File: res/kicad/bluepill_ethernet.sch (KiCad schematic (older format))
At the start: 12 parts, among them J2 Conn_01x03, U1 BluePill_STM32F103C, U2 93C46, U3 WIZ850io

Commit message: Add button to kicad circuit for 'factory reset' the configuration (delete eeprom)
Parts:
- added SW?: SW_Push, symbol switches:SW_Push
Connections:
- wire segments 100 -> 104
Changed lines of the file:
@@
 	5600 1200 5600 1500
+Wire Wire Line
+	3050 900  2450 900
 Wire Wire Line
 	3050 900  3750 900
@@
 Wire Wire Line
 	4300 2350 4300 2550
-Wire Wire Line
-	2150 900  3050 900
+$Comp
+L switches:SW_Push SW?
+U 1 1 5ADFA2DD
+P 2450 2500
+F 0 "SW?" V 2404 2648 50  0000 L CNN
+F 1 "SW_Push" V 2495 2648 50  0000 L CNN
+F 2 "" H 2450 2700 50  0001 C CNN
+F 3 "" H 2450 2700 50  0001 C CNN
+	1    2450 2500
+	0    1    1    0
+$EndComp
+Wire Wire Line
+	2550 2950 2450 2950
+Wire Wire Line
+	2450 2950 2450 2700
+Wire Wire Line
+	2450 2300 2450 900
+Connection ~ 2450 900
+Wire Wire Line
+	2450 900  2150 900
 $EndSCHEMATC

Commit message: Revision 2.0
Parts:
- added D1, D2, D3: LED, LEDs:LED_D3.0mm, symbol device:LED
- added J1: HEADER-1x20, Pin_Headers:Pin_Header_Straight_1x20_Pitch2.54mm, symbol connectors:HEADER-1x20
- added R2, R3, R4, R5, R6: R, Resistors_THT:R_Axial_DIN0204_L3.6mm_D1.6mm_P5.08mm_Horizontal, symbol device:R
- SW1: renamed from SW?; footprint (none) -> Buttons_Switches_THT:SW_PUSH_6mm
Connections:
- wire segments 104 -> 125
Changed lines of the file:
@@
 	4300 2350 4300 2550
 $Comp
-L switches:SW_Push SW?
+L switches:SW_Push SW1
 U 1 1 5ADFA2DD
 P 2450 2500
-F 0 "SW?" V 2404 2648 50  0000 L CNN
+F 0 "SW1" V 2404 2648 50  0000 L CNN
 F 1 "SW_Push" V 2495 2648 50  0000 L CNN
-F 2 "" H 2450 2700 50  0001 C CNN
+F 2 "Buttons_Switches_THT:SW_PUSH_6mm" H 2450 2700 50  0001 C CNN
 F 3 "" H 2450 2700 50  0001 C CNN
 	1    2450 2500
@@
 Wire Wire Line
 	2450 900  2150 900
+$Comp
+L connectors:HEADER-1x20 J1
+U 1 1 5B103221
+P 4450 3500
+F 0 "J1" H 4578 3536 60  0000 L CNB
+F 1 "HEADER-1x20" H 4578 3445 40  0000 L CNN
+F 2 "Pin_Headers:Pin_Header_Straight_1x20_Pitch2.54mm" H 4450 3500 60  0001 C CNN
+F 3 "" H 4450 3500 60  0001 C CNN
+F 4 "-" H 4400 4650 40  0001 L BNN "Part"
+F 5 "Connector" H 4400 4750 40  0001 L BNN "Family"
+	1    4450 3500
+	1    0    0    -1
+$EndComp
+Connection ~ 4300 2550
+Connection ~ 4300 2650
+Connection ~ 4300 2750
+$Comp
+L device:R R3
+U 1 1 5B105160
+P 3600 2850
+F 0 "R3" V 3680 2850 50  0000 C CNN
+F 1 "R" V 3600 2850 50  0000 C CNN
+F 2 "Resistors_THT:R_Axial_DIN0204_L3.6mm_D1.6mm_P5.08mm_Horizontal" V 3530 2850 50  0001 C CNN
+F 3 "" H 3600 2850 50  0001 C CNN
+	1    3600 2850
+	1    0    0    -1
+$EndComp
+$Comp
+L device:R R2
+U 1 1 5B105A17
+P 3500 2850
+F 0 "R2" V 3580 2850 50  0000 C CNN
+F 1 "R" V 3500 2850 50  0000 C CNN
+F 2 "Resistors_THT:R_Axial_DIN0204_L3.6mm_D1.6mm_P5.08mm_Horizontal" V 3430 2850 50  0001 C CNN
+F 3 "" H 3500 2850 50  0001 C CNN
+	1    3500 2850
+	1    0    0    -1
+$EndComp
+Wire Wire Line
+	3600 3050 3600 3000
+Wire Wire Line
+	3500 3150 3500 3000
+Wire Wire Line
+	4300 2550 3600 2550
+Wire Wire Line
+	3600 2550 3600 2700
+Wire Wire Line
+	3500 2700 3500 2550
+Wire Wire Line
+	3500 2550 3600 2550
+Connection ~ 3600 2550
+Wire Wire Line
+	3600 3050 4300 3050
+Connection ~ 4300 3050
+Wire Wire Line
+	3500 3150 4300 3150
+Connection ~ 4300 3150
+$Comp
+L device:LED D1
+U 1 1 5B11D9D9
+P 1100 4350
+F 0 "D1" V 1138 4233 50  0000 R CNN
+F 1 "LED" V 1047 4233 50  0000 R CNN
+F 2 "LEDs:LED_D3.0mm" H 1100 4350 50  0001 C CNN
+F 3 "" H 1100 4350 50  0001 C CNN
+	1    1100 4350
+	0    -1   -1   0
+$EndComp
+$Comp
+L device:LED D2
+U 1 1 5B11DDF6
+P 1350 4350
+F 0 "D2" V 1388 4233 50  0000 R CNN
+F 1 "LED" V 1297 4233 50  0000 R CNN
+F 2 "LEDs:LED_D3.0mm" H 1350 4350 50  0001 C CNN
+F 3 "" H 1350 4350 50  0001 C CNN
+	1    1350 4350
+	0    -1   -1   0
+$EndComp
+$Comp
+L device:LED D3
+U 1 1 5B11DE60
+P 1550 4350
+F 0 "D3" V 1588 4233 50  0000 R CNN
+F 1 "LED" V 1497 4233 50  0000 R CNN
+F 2 "LEDs:LED_D3.0mm" H 1550 4350 50  0001 C CNN
+F 3 "" H 1550 4350 50  0001 C CNN
+	1    1550 4350
+	0    -1   -1   0
+$EndComp
+Wire Wire Line
+	2550 3050 1100 3050
+Wire Wire Line
+	1100 3050 1100 4200
+Wire Wire Line
+	2550 3150 1350 3150
+Wire Wire Line
+	1350 3150 1350 4200
+Wire Wire Line
+	2550 3250 1550 3250
+Wire Wire Line
+	1550 3250 1550 4200
+$Comp
+L device:R R4
+U 1 1 5B129B3F
+P 1100 4650
+F 0 "R4" V 1180 4650 50  0000 C CNN
+F 1 "R" V 1100 4650 50  0000 C CNN
+F 2 "Resistors_THT:R_Axial_DIN0204_L3.6mm_D1.6mm_P5.08mm_Horizontal" V 1030 4650 50  0001 C CNN
+F 3 "" H 1100 4650 50  0001 C CNN
+	1    1100 4650
+	1    0    0    -1
+$EndComp
+$Comp
+L device:R R5
+U 1 1 5B129C2D
+P 1350 4650
+F 0 "R5" V 1430 4650 50  0000 C CNN
+F 1 "R" V 1350 4650 50  0000 C CNN
+F 2 "Resistors_THT:R_Axial_DIN0204_L3.6mm_D1.6mm_P5.08mm_Horizontal" V 1280 4650 50  0001 C CNN
+F 3 "" H 1350 4650 50  0001 C CNN
+	1    1350 4650
+	1    0    0    -1
+$EndComp
+$Comp
+L device:R R6
+U 1 1 5B129C71
+P 1550 4650
+F 0 "R6" V 1630 4650 50  0000 C CNN
+F 1 "R" V 1550 4650 50  0000 C CNN
+F 2 "Resistors_THT:R_Axial_DIN0204_L3.6mm_D1.6mm_P5.08mm_Horizontal" V 1480 4650 50  0001 C CNN
+F 3 "" H 1550 4650 50  0001 C CNN
+	1    1550 4650
+	1    0    0    -1
+$EndComp
+Wire Wire Line
+	2550 4550 2550 5850
+Wire Wire Line
+	2550 5850 1550 5850
+Wire Wire Line
+	1100 5850 1100 4800
+Connection ~ 2550 4550
+Wire Wire Line
+	1350 4800 1350 5850
+Connection ~ 1350 5850
+Wire Wire Line
+	1350 5850 1100 5850
+Wire Wire Line
+	1550 4800 1550 5850
+Connection ~ 1550 5850
+Wire Wire Line
+	1550 5850 1350 5850
 $EndSCHEMATC

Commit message: Fix production issues (also add molex pin for other W5500 boards)
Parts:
- added J3: Conn_02x05_Odd_Even, Pin_Headers:Pin_Header_Straight_2x05_Pitch2.54mm, symbol conn:Conn_02x05_Odd_Even
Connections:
- wire segments 125 -> 148
- no-connect marks 0 -> 3
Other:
- moved on the sheet: J1, U1, U2, U3

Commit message: board revision 3 alpha 1
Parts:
- removed C3: C, Capacitors_THT:C_Disc_D3.0mm_W2.0mm_P2.50mm, symbol device:C
- added J4: HEADER-1x20, Pin_Headers:Pin_Header_Straight_1x20_Pitch2.54mm, symbol connectors:HEADER-1x20
- added U4: 93C46, Housings_SSOP:TSSOP-8_4.4x3mm_Pitch0.65mm, symbol 93c46:93C46
- C1, C5, C7: footprint Capacitors_THT:C_Disc_D3.0mm_W2.0mm_P2.50mm -> Capacitors_THT:C_Disc_D4.3mm_W1.9mm_P5.00mm; symbol device:C -> bluepill_ethernet-rescue:C-device
- C2, C4, C6: symbol device:CP -> bluepill_ethernet-rescue:CP-device
- D1, D2, D3: symbol device:LED -> bluepill_ethernet-rescue:LED-device
- J2: symbol conn:Conn_01x03 -> bluepill_ethernet-rescue:Conn_01x03-conn
- J3: symbol conn:Conn_02x05_Odd_Even -> bluepill_ethernet-rescue:Conn_02x05_Odd_Even-conn
- R1, R2, R3, R4, R5, R6: footprint Resistors_THT:R_Axial_DIN0204_L3.6mm_D1.6mm_P5.08mm_Horizontal -> Resistors_Universal:Resistor_SMD+THTuniversal_0805to1206_RM10_HandSoldering; symbol device:R -> bluepill_ethernet-rescue:R-device
- SW1: symbol switches:SW_Push -> bluepill_ethernet-rescue:SW_Push-switches
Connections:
- wire segments 148 -> 150
- no-connect marks 3 -> 5
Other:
- moved on the sheet: J1, U1, U2, U3

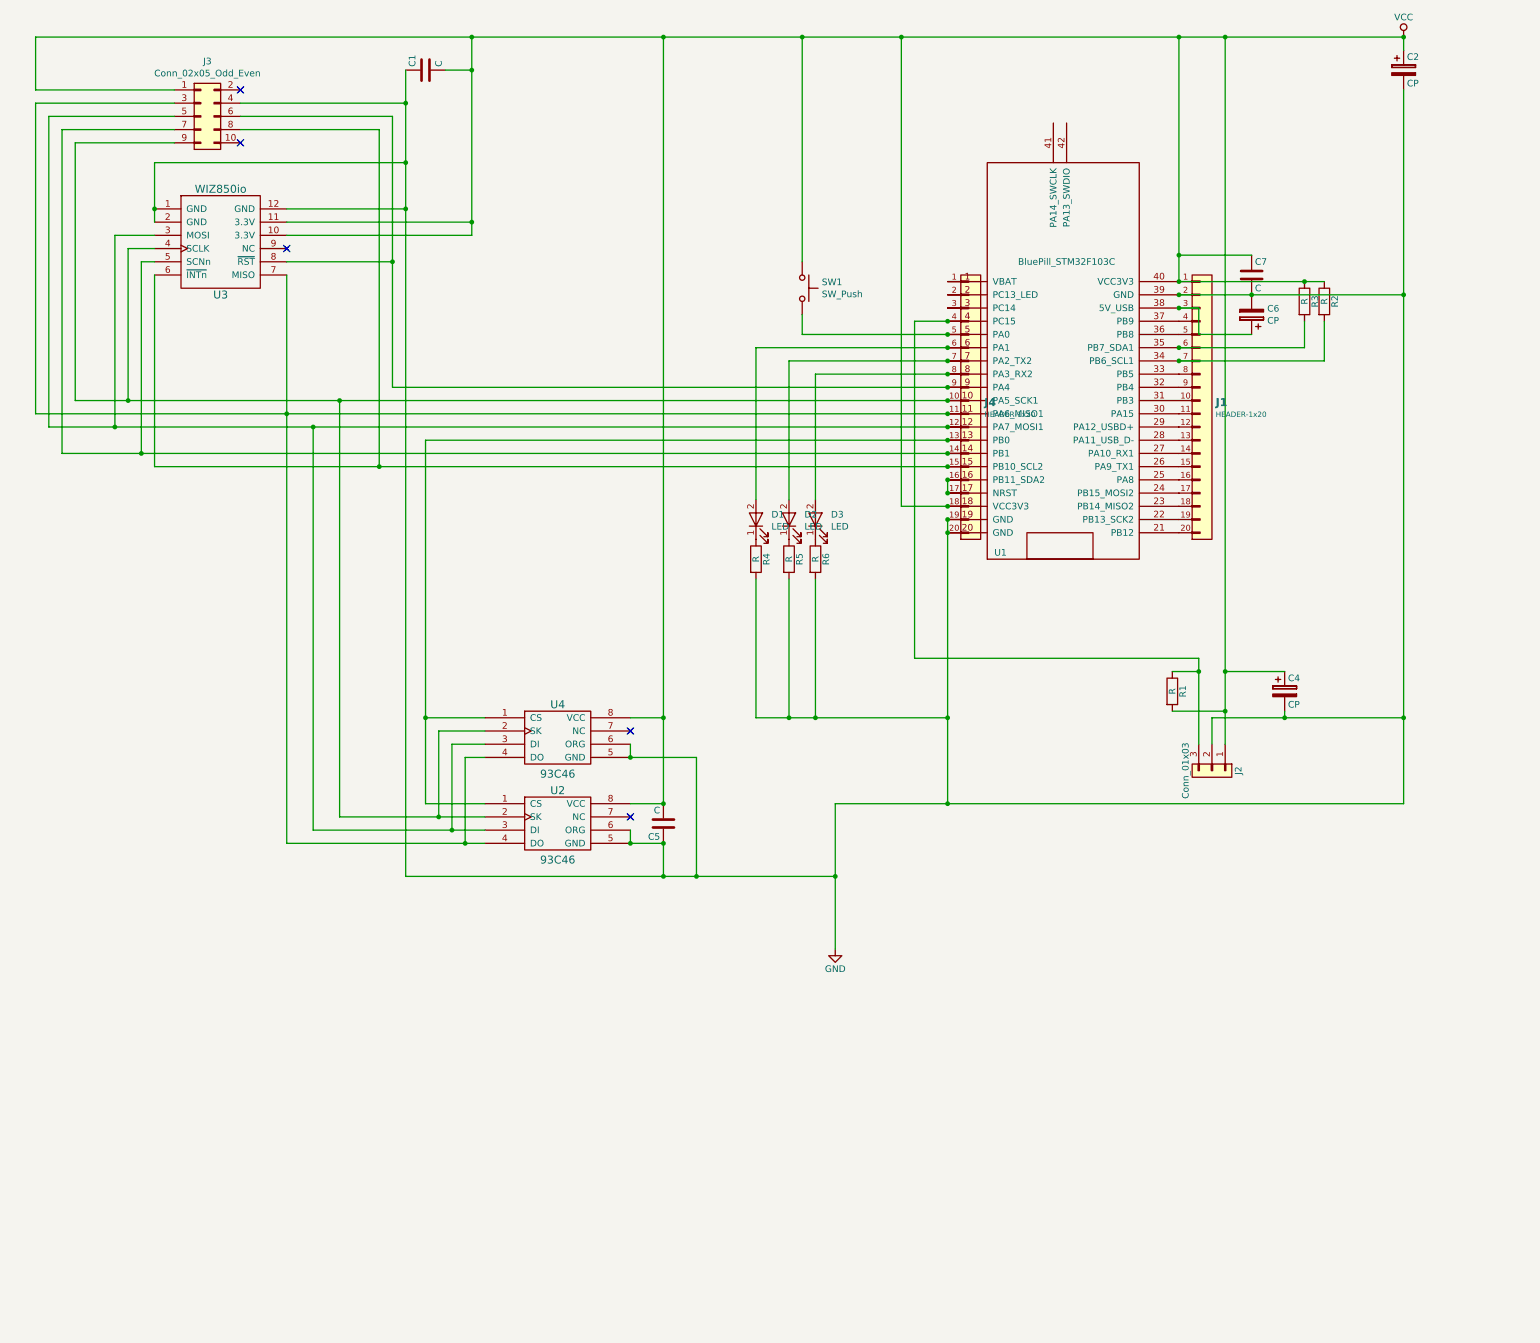
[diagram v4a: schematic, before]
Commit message: Board Rev 3.0
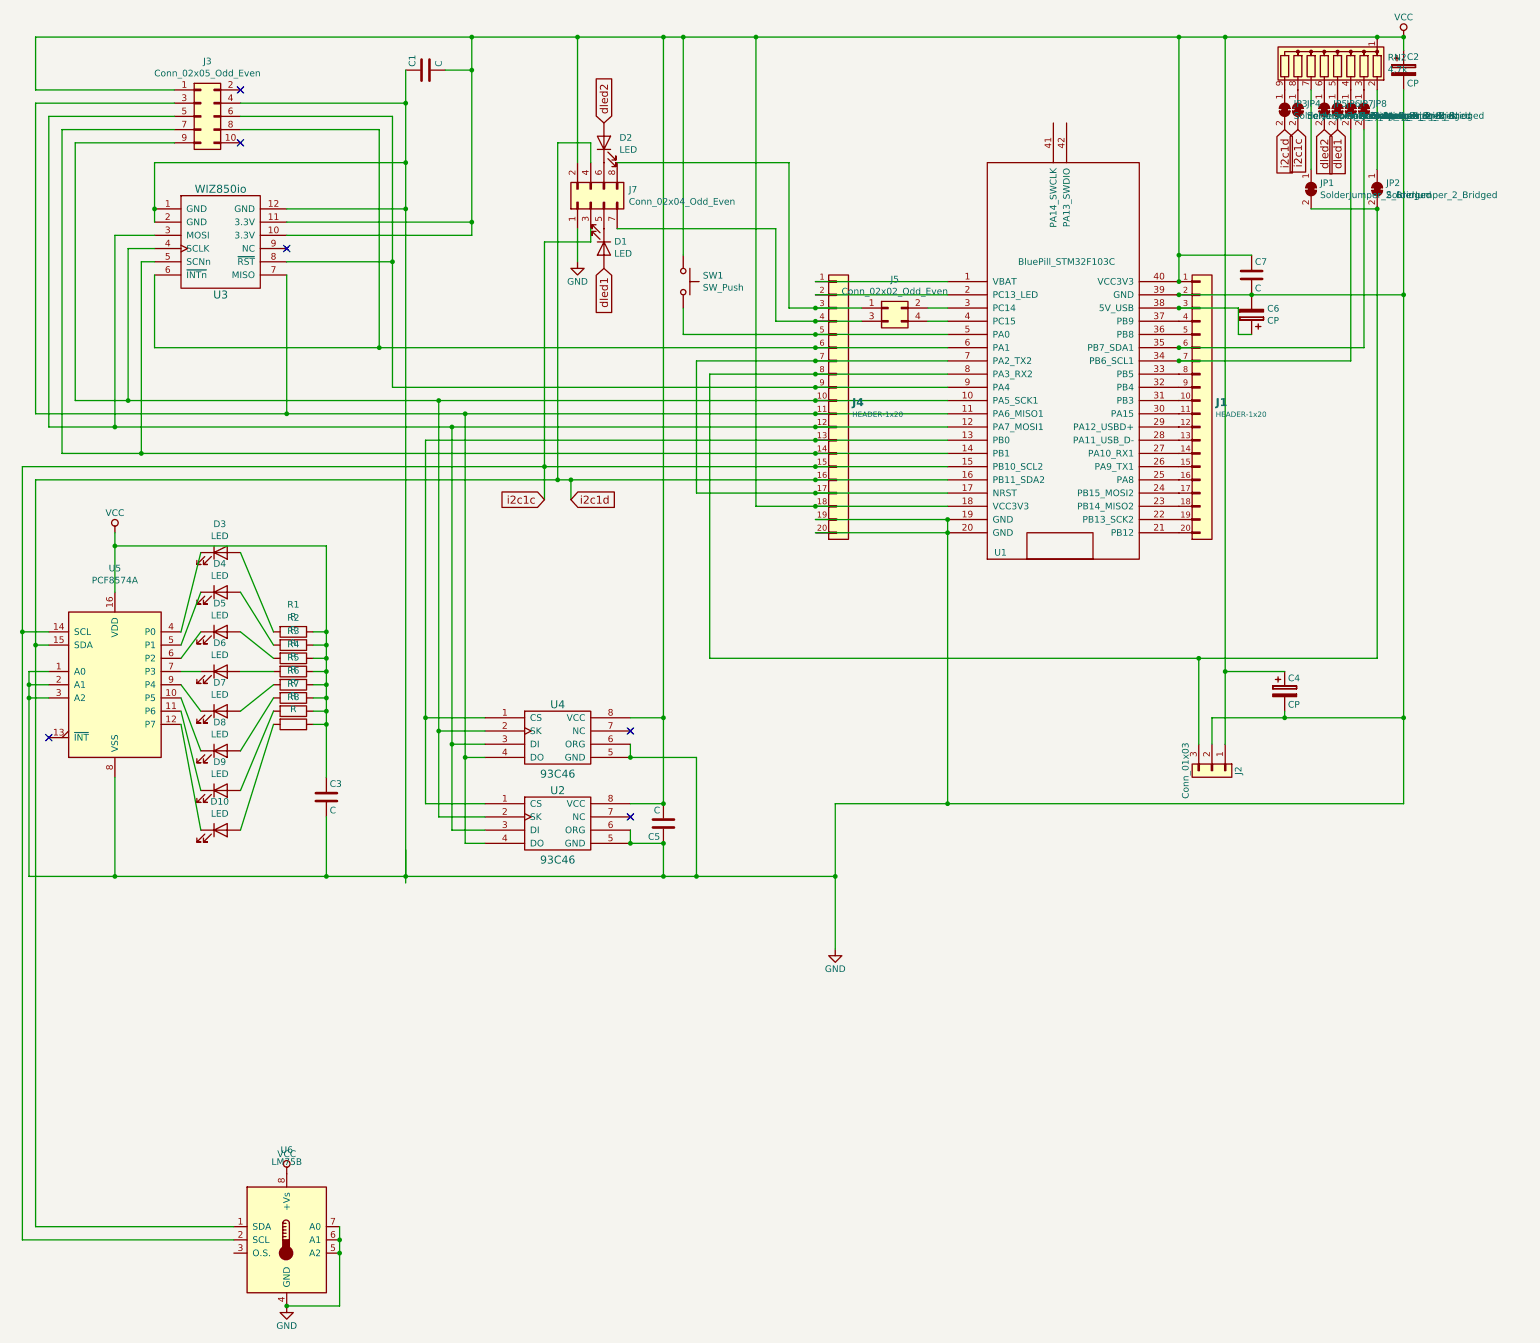
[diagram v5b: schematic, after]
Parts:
- removed D1, D2, D3: LED, LEDs:LED_D3.0mm, symbol bluepill_ethernet-rescue:LED-device
- removed R1, R2, R3, R4, R5, R6: R, Resistors_Universal:Resistor_SMD+THTuniversal_0805to1206_RM10_HandSoldering, symbol bluepill_ethernet-rescue:R-device
- added C3: C, Capacitor_SMD:C_0805_2012Metric, symbol bluepill_ethernet-rescue:C-device
- added D1, D2: LED, LED_THT:LED_D3.0mm, symbol Device:LED
- added D10, D3, D4, D5, D6, D7, D8, D9: LED, LED_SMD:LED_1206_3216Metric, symbol Device:LED
- added J5: Conn_02x02_Odd_Even, Connector_PinHeader_2.54mm:PinHeader_2x02_P2.54mm_Vertical, symbol Connector_Generic:Conn_02x02_Odd_Even
- added J7: Conn_02x04_Odd_Even, Connector_PinHeader_2.54mm:PinHeader_2x04_P2.54mm_Vertical, symbol Connector_Generic:Conn_02x04_Odd_Even
- added JP1, JP2, JP3, JP4, JP5, JP6, JP7, JP8: SolderJumper_2_Bridged, Jumper:SolderJumper-2_P1.3mm_Bridged_RoundedPad1.0x1.5mm, symbol Jumper:SolderJumper_2_Bridged
- added R1, R2, R3, R4, R5, R6, R7, R8: R, Resistor_SMD:R_0805_2012Metric, symbol Device:R
- added RN2: 4,7k, Resistor_THT:R_Array_SIP9, symbol Device:R_Network08
- added U5: PCF8574A, Package_SO:TSSOP-20_4.4x6.5mm_P0.65mm, symbol Interface_Expansion:PCF8574A
- added U6: LM75B, Package_SO:VSSOP-8_3.0x3.0mm_P0.65mm, symbol Sensor_Temperature:LM75B
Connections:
- net GND: now also C3.2, J7.1 (Pin_1), U5.1 (A0), U5.2 (A1), U5.3 (A2), U5.8 (VSS), U6.4 (GND), U6.5 (A2), U6.6 (A1), U6.7 (A0)
- net VCC: now also C3.1, J7.2 (Pin_2), R1.1, R2.1, R3.1, R4.1, R5.1, R6.1, R7.1, R8.1, RN2.1 (common), U5.16 (VDD), U6.8 (+Vs)
- net at J3.8 (Pin_8), U3.6 (~INTn): now also J4.6 (P6), U1.6 (PA1); no longer J4.15 (P15), U1.15 (PB10_SCL2)
- net at J4.17 (P17), U1.17 (NRST): now also J4.7 (P7), U1.7 (PA2_TX2); no longer J4.16 (P16), U1.16 (PB11_SDA2)
- net at U1.3 (PC14): now also J5.2 (Pin_2); no longer J4.3 (P3)
- net at J1.7 (P7), U1.34 (PB6_SCL1): now also JP7.2 (B)
- net at J1.6 (P6), U1.35 (PB7_SDA1): now also JP8.2 (B)
- net at J4.8 (P8), U1.8 (PA3_RX2): now also J2.3 (Pin_3), JP1.2 (B), JP2.2 (B)
- new net: J5.4 (Pin_4), U1.4 (PC15)
- new net: D4.1 (K), U5.5 (P1)
- new net: D4.2 (A), R2.2
- new net: D8.1 (K), U5.10 (P5)
- new net: D9.1 (K), U5.11 (P6)
- new net: D10.1 (K), U5.12 (P7)
- new net: D3.1 (K), U5.4 (P0)
- new net: D5.1 (K), U5.6 (P2)
- new net: D6.1 (K), U5.7 (P3)
- new net: D7.1 (K), U5.9 (P4)
- new net: J4.3 (P3), J5.1 (Pin_1), J7.8 (Pin_8)
- new net: J4.4 (P4), J5.3 (Pin_3), J7.7 (Pin_7)
- new net: JP2.1 (A), RN2.2 (R1)
- new net: JP8.1 (A), RN2.3 (R2)
- new net: JP7.1 (A), RN2.4 (R3)
- new net: JP6.1 (A), RN2.5 (R4)
- new net: JP5.1 (A), RN2.6 (R5)
- new net: JP1.1 (A), RN2.7 (R6)
- new net: JP4.1 (A), RN2.8 (R7)
- new net: JP3.1 (A), RN2.9 (R8)
- new net: D2.1 (K), J7.6 (Pin_6)
- new net: D1.1 (K), J7.5 (Pin_5)
- new net: D3.2 (A), R1.2
- new net: D5.2 (A), R3.2
- new net: D6.2 (A), R4.2
- new net: D7.2 (A), R5.2
- new net: D8.2 (A), R6.2
- new net: D9.2 (A), R7.2
- new net: D10.2 (A), R8.2
- new net dled1: D1.2 (A), JP6.2 (B)
- new net dled2: D2.2 (A), JP5.2 (B)
- new net i2c1c: J4.15 (P15), J7.3 (Pin_3), JP4.2 (B), U1.15 (PB10_SCL2), U5.14 (SCL), U6.2 (SCL)
- new net i2c1d: J4.16 (P16), J7.4 (Pin_4), JP3.2 (B), U1.16 (PB11_SDA2), U5.15 (SDA), U6.1 (SDA)
- no-connect marks 5 -> 6
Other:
- moved on the sheet: J4, SW1

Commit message: Board rev 3.1: Fix invalid pcf8574 footprint (20->16 pins)
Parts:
- U5: footprint Package_SO:TSSOP-20_4.4x6.5mm_P0.65mm -> Package_SO:TSSOP-16_4.4x5mm_P0.65mm
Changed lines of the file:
@@
 F 0 "U5" H 1300 6431 50  0000 C CNN
 F 1 "PCF8574A" H 1300 6340 50  0000 C CNN
-F 2 "Package_SO:TSSOP-20_4.4x6.5mm_P0.65mm" H 1300 5550 50  0001 C CNN
+F 2 "Package_SO:TSSOP-16_4.4x5mm_P0.65mm" H 1300 5550 50  0001 C CNN
 F 3 "http://www.nxp.com/documents/data_sheet/PCF8574_PCF8574A.pdf" H 1300 5550 50  0001 C CNN
 	1    1300 5550

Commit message: Replace TSSOP packages with SOIC packages
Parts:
- U4: footprint Housings_SSOP:TSSOP-8_4.4x3mm_Pitch0.65mm -> Package_SO:SOIC-8_5.23x5.23mm_P1.27mm
- U5: footprint Package_SO:TSSOP-16_4.4x5mm_P0.65mm -> Package_SO:SOIC-16W_7.5x10.3mm_P1.27mm
- U6: footprint Package_SO:VSSOP-8_3.0x3.0mm_P0.65mm -> Package_SO:SOIC-8_3.9x4.9mm_P1.27mm
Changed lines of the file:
@@
 F 0 "U4" H 4650 6200 60  0000 C CNN
 F 1 "93C46" H 4650 5675 60  0000 C CNN
-F 2 "Housings_SSOP:TSSOP-8_4.4x3mm_Pitch0.65mm" H 4650 5950 60  0001 C CNN
+F 2 "Package_SO:SOIC-8_5.23x5.23mm_P1.27mm" H 4650 5950 60  0001 C CNN
 F 3 "" H 4650 5950 60  0001 C CNN
 	1    4650 5950
@@
 F 0 "U5" H 1300 6431 50  0000 C CNN
 F 1 "PCF8574A" H 1300 6340 50  0000 C CNN
-F 2 "Package_SO:TSSOP-16_4.4x5mm_P0.65mm" H 1300 5550 50  0001 C CNN
+F 2 "Package_SO:SOIC-16W_7.5x10.3mm_P1.27mm" H 1300 5550 50  0001 C CNN
 F 3 "http://www.nxp.com/documents/data_sheet/PCF8574_PCF8574A.pdf" H 1300 5550 50  0001 C CNN
 	1    1300 5550
@@
 F 0 "U6" H 2600 10431 50  0000 C CNN
 F 1 "LM75B" H 2600 10340 50  0000 C CNN
-F 2 "Package_SO:VSSOP-8_3.0x3.0mm_P0.65mm" H 2600 9750 50  0001 C CNN
+F 2 "Package_SO:SOIC-8_3.9x4.9mm_P1.27mm" H 2600 9750 50  0001 C CNN
 F 3 "http://www.ti.com/lit/ds/symlink/lm75b.pdf" H 2600 9750 50  0001 C CNN
 	1    2600 9750
